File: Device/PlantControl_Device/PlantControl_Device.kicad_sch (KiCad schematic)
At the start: 19 parts, among them J2 Power, U1 NRF24L01_Breakout, U2 PIC18F15Q41-I/SS, U3 AHT20, U4 BH1750FVI-TR, U5 NCP1117-3.3Vout-20Vin

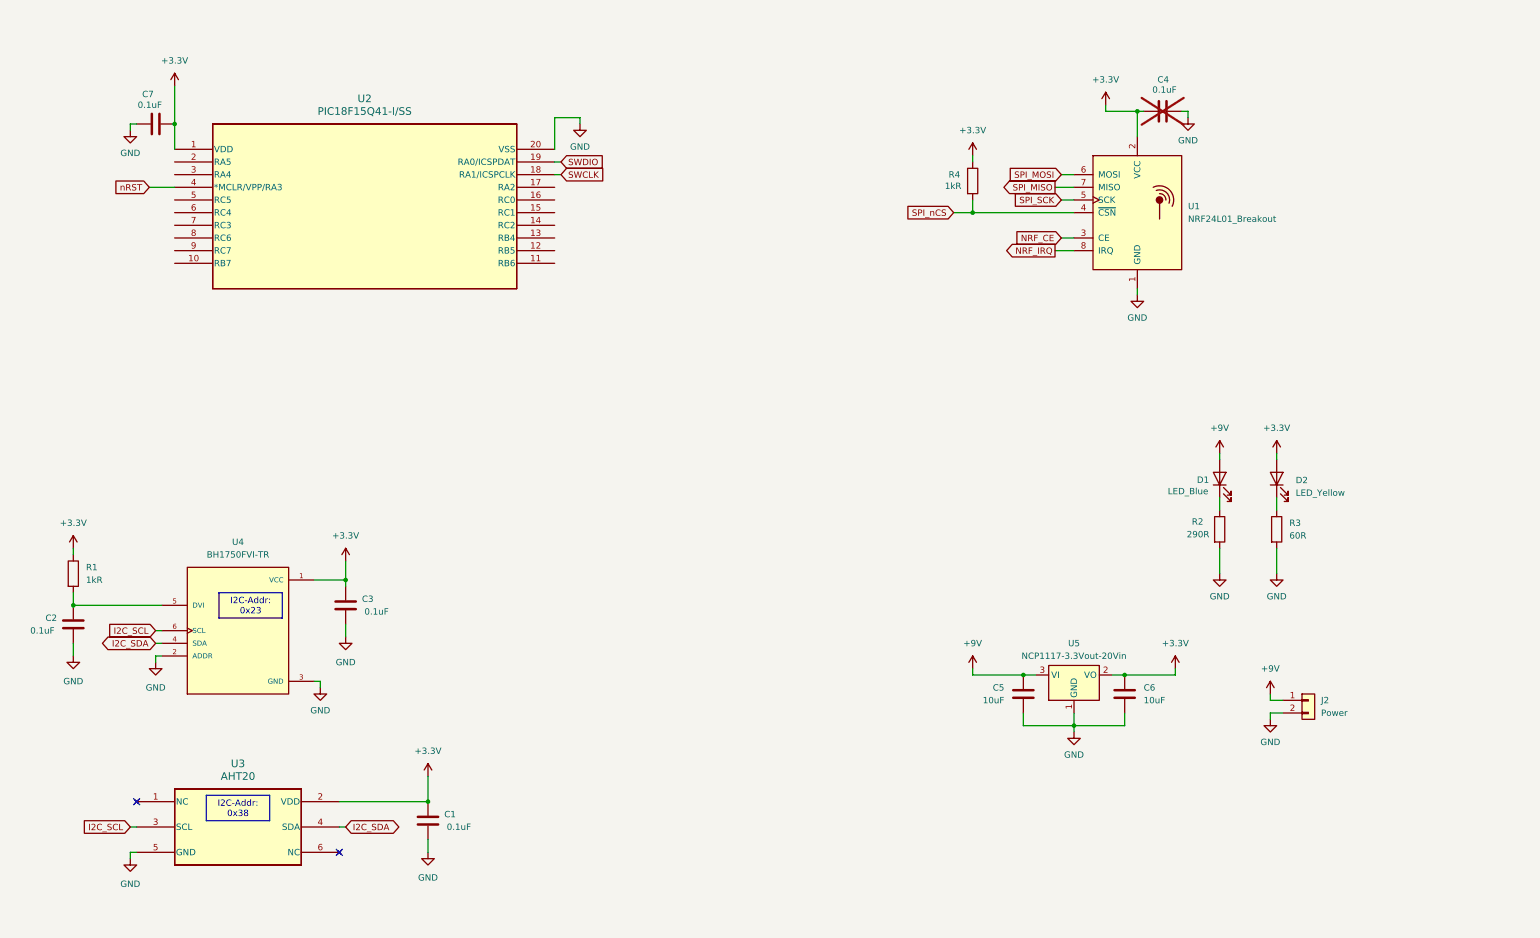
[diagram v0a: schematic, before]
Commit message: First layout
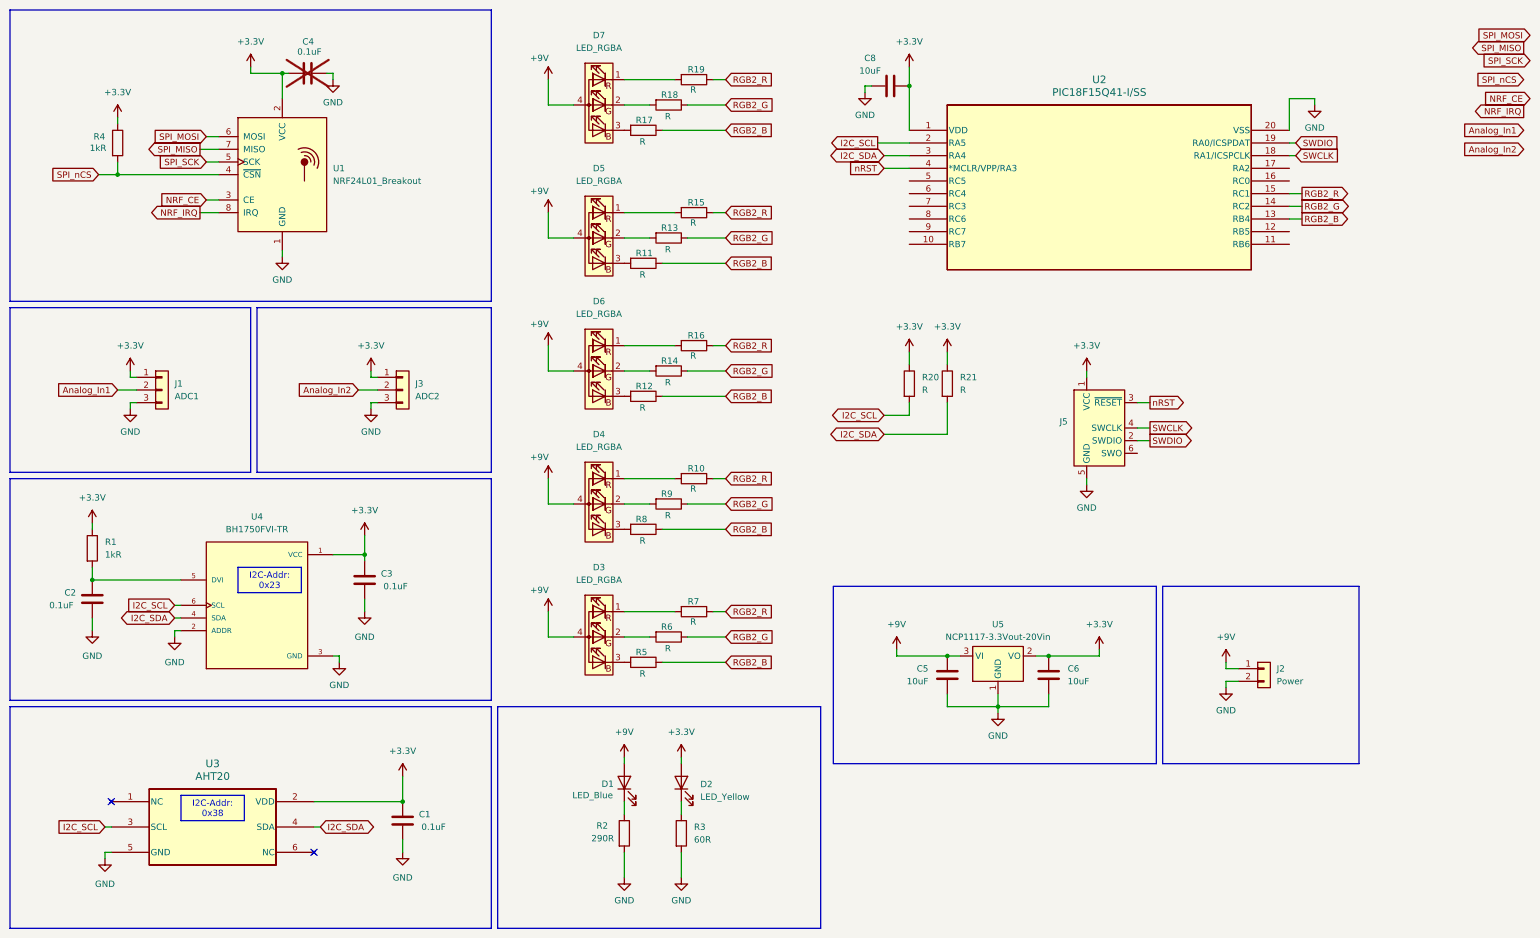
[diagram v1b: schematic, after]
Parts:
- removed C7: 0.1uF, Capacitor_SMD:C_0805_2012Metric_Pad1.18x1.45mm_HandSolder, symbol Device:C
- added C8: 10uF, Capacitor_THT:C_Disc_D4.3mm_W1.9mm_P5.00mm, symbol Device:C
- added D3, D4, D5, D6, D7: LED_RGBA, cr_Library:cr_RGB_LED, symbol Device:LED_RGBA
- added J1: ADC1, Connector_PinHeader_2.00mm:PinHeader_1x03_P2.00mm_Vertical, symbol Connector_Generic:Conn_01x03
- added J3: ADC2, Connector_PinHeader_2.00mm:PinHeader_1x03_P2.00mm_Vertical, symbol Connector_Generic:Conn_01x03
- added J5: Conn_ARM_SWD_TagConnect_TC2030-NL, Connector:Tag-Connect_TC2030-IDC-NL_2x03_P1.27mm_Vertical, symbol Connector:Conn_ARM_SWD_TagConnect_TC2030-NL
- added R10, R11, R12, R13, R14, R15, R16, R17, R18, R19, R5, R6, R7, R8, R9: R, Resistor_THT:R_Axial_DIN0207_L6.3mm_D2.5mm_P7.62mm_Horizontal, symbol Device:R
- added R20, R21: R, Resistor_SMD:R_0805_2012Metric_Pad1.20x1.40mm_HandSolder, symbol Device:R
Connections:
- net +3.3V: now also C8.2, J1.1 (Pin_1), J3.1 (Pin_1), J5.1 (VCC), R20.1, R21.1
- net +9V: now also D3.4 (A), D4.4 (A), D5.4 (A), D6.4 (A), D7.4 (A)
- net GND: now also C8.1, J1.3 (Pin_3), J3.3 (Pin_3), J5.5 (GND)
- net I2C_SCL: now also U2.2 (RA5), R20.2
- net I2C_SDA: now also U2.3 (RA4), R21.2
- net SWCLK: now also J5.4 (SWCLK)
- net SWDIO: now also J5.2 (SWDIO)
- net nRST: now also J5.3 (~{RESET})
- net RGB2_B: now reaches U2.13 (RB4)
- net RGB2_B: now also R11.1, R12.1, R17.1, R5.1, R8.1
- net RGB2_G: now reaches U2.14 (RC2)
- net RGB2_G: now also R13.1, R14.1, R18.1, R6.1, R9.1
- net RGB2_R: now reaches U2.15 (RC1)
- net RGB2_R: now also R10.1, R15.1, R16.1, R19.1, R7.1
- new net: D5.1 (RK), R15.2
- new net: D5.2 (GK), R13.2
- new net: D5.3 (BK), R11.2
- new net: D4.1 (RK), R10.2
- new net: D4.2 (GK), R9.2
- new net: D4.3 (BK), R8.2
- new net: D6.1 (RK), R16.2
- new net: D6.2 (GK), R14.2
- new net: D6.3 (BK), R12.2
- new net: D7.1 (RK), R19.2
- new net: D7.2 (GK), R18.2
- new net: D7.3 (BK), R17.2
- new net: D3.1 (RK), R7.2
- new net: D3.2 (GK), R6.2
- new net: D3.3 (BK), R5.2
- new net Analog_In1: J1.2 (Pin_2)
- new net Analog_In2: J3.2 (Pin_2)
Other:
- moved on the sheet: C1, C2, C3, C4, C5, C6, D1, D2, J2, R1, R2, R3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
